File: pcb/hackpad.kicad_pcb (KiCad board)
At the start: 2 copper layers, 90.7 x 57.3 mm, 19 parts, among them SW1 RotaryEncoder_Switch, SW2 SW_Push, SW3 SW_Push, SW4 SW_Push, SW5 SW_Push, SW6 SW_Push, SW7 SW_Push, SW8 SW_Push, SW9 SW_Push, U1 MOUDLE-SEEEDUINO-XIAO, U2 ER_OLEDM0.91_1x-I2C

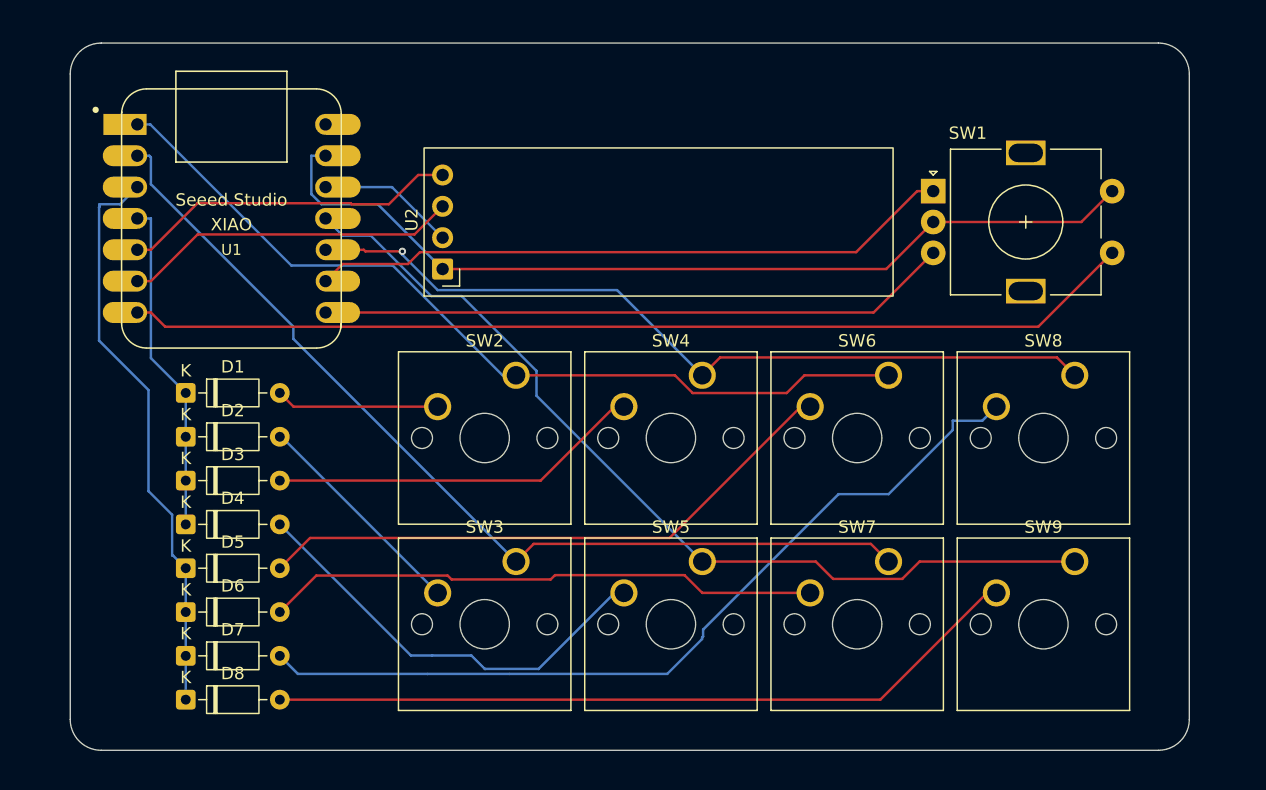
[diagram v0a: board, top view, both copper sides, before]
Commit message: Added case modeling files (WIP)
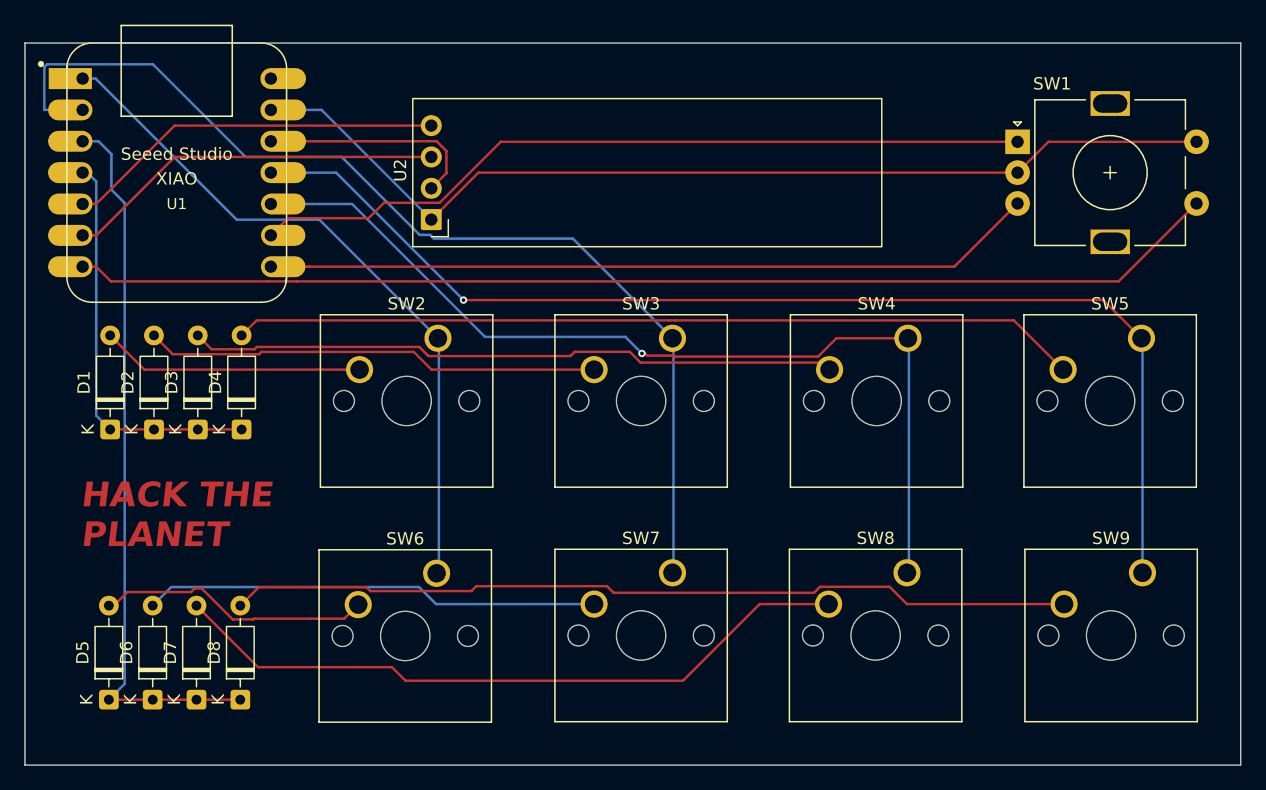
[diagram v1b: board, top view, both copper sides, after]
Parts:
- moved SW6 40.0 mm to (134.3, 114.5)
- moved SW5 39.9 mm to (191.5, 95.4)
- moved SW3 22.1 mm to (153.5, 95.4)
- moved SW8 21.0 mm to (172.5, 114.4)
- moved SW7 17.5 mm to (153.5, 114.4)
- moved SW4 16.9 mm to (172.5, 95.4)
- moved D5 12.3 mm to (107.8, 124.7), turned to 90 degrees
- moved D4 8.92 mm to (118.5, 102.8), turned to 90 degrees
- moved SW1 7.92 mm to (181.4, 79.5)
- moved D6 7.59 mm to (111.3, 124.7), turned to 90 degrees
- moved SW2 7.00 mm to (134.5, 95.4)
- moved D1 6.80 mm to (107.9, 102.8), turned to 90 degrees
- moved U1 5.78 mm to (113.3, 82.0)
- moved SW9 5.56 mm to (191.5, 114.4)
- moved D8 4.42 mm to (118.4, 124.7), turned to 90 degrees
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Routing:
- net Net-(D4-A): track 35.3 -> 68.7 mm
- net Net-(D5-A): track 48.4 -> 22.3 mm
- net Net-(D3-A): track 30.4 -> 52.8 mm
- net /COL4: track 74.6 -> 95.1 mm, vias 0 -> 1
- net Net-(D2-A): track 18.0 -> 37.0 mm
- net /COL1: track 70.5 -> 56.7 mm
- net Net-(D7-A): track 68.5 -> 56.3 mm
- net /ROW2: track 46.7 -> 58.6 mm
- net Net-(U1-PB08_A6_D6_TX): track 81.9 -> 93.4 mm
- net Net-(U1-PB09_A7_D7_RX): track 51.2 -> 62.6 mm
- net Net-(U1-PA7_A8_D8_SCK): track 52.3 -> 63.6 mm
- net /COL3: track 66.3 -> 76.5 mm
- net /COL2: track 77.5 -> 85.8 mm
- net Net-(D1-A): track 13.2 -> 21.4 mm
- net Net-(D6-A): track 45.1 -> 37.0 mm
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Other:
- board size 90.7 x 57.3 mm -> 98.5 x 58.5 mm
- board text added: "HACK THE PLANET"
